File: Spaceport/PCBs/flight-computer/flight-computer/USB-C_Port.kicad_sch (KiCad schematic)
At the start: 4 parts, among them J4 USB_C_Receptacle_USB2.0_16P

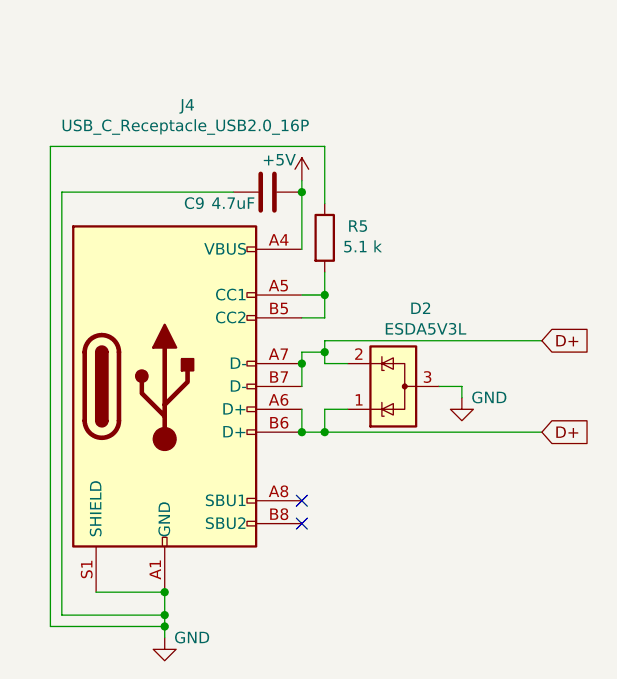
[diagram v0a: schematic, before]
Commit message: removed SdCard
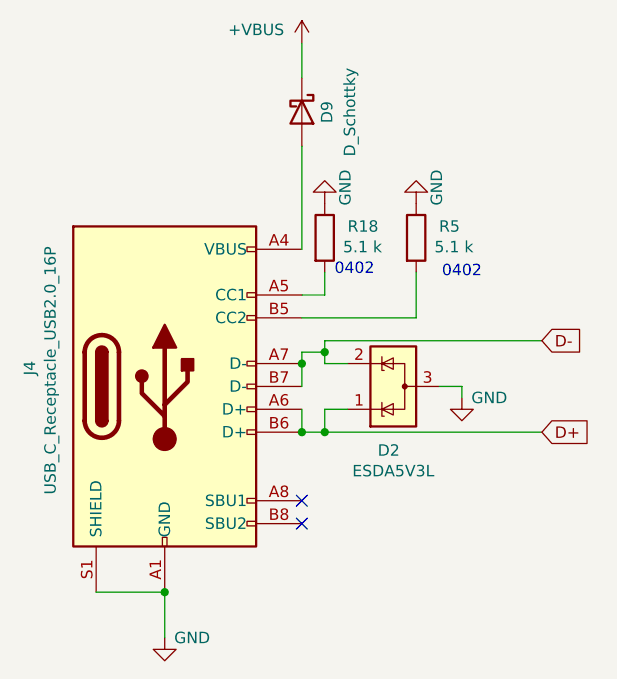
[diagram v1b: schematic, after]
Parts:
- removed C9: 4.7uF, symbol Device:C
- added D9: D_Schottky, symbol Device:D_Schottky
- added R18: 5.1 k, symbol Device:R
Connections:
- net D+: no longer D2.2 (K), J4.A7 (D-), J4.B7 (D-)
- net GND: now also R18.1
- net at J4.B5 (CC2), R5.2: no longer J4.A5 (CC1)
- net +5V: no longer names the net of J4.A4 (VBUS), J4.A9 (VBUS), J4.B4 (VBUS), J4.B9 (VBUS)
- net +5V: now also D9.2 (A)
- new net: J4.A5 (CC1), R18.2
- new net +VBUS: D9.1 (K)
- new net D-: D2.2 (K), J4.A7 (D-), J4.B7 (D-)
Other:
- note added: "0402"
- moved on the sheet: R5

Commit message: added footprints and fixed 3.3v/gnd connector orientation
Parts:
- D9: footprint (none) -> Diode_SMD:D_0805_2012Metric_Pad1.15x1.40mm_HandSolder
- R18, R5: footprint (none) -> Resistor_SMD:R_0603_1608Metric_Pad0.98x0.95mm_HandSolder
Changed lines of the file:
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@@
 			)
 		)
-		(property "Footprint" ""
+		(property "Footprint" "Diode_SMD:D_0805_2012Metric_Pad1.15x1.40mm_HandSolder"
 			(at 132.08 68.58 0)
 			(effects
@@
 			)
 		)
-		(property "Footprint" ""
+		(property "Footprint" "Resistor_SMD:R_0603_1608Metric_Pad0.98x0.95mm_HandSolder"
 			(at 132.842 82.55 90)
 			(effects
@@
 			)
 		)
-		(property "Footprint" ""
+		(property "Footprint" "Resistor_SMD:R_0603_1608Metric_Pad0.98x0.95mm_HandSolder"
 			(at 143.002 82.55 90)
 			(effects
